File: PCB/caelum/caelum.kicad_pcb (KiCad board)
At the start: 2 copper layers, 48 x 37 mm, 18 parts, among them J1 BATT+, J2 BATT-, J5 PulseIN, J6 PulseOUT, J7 Conn_01x04_Pin, Q1 FS8205A, U1 DW01A, U2 MCP1700T-3302E, U3 ESP32-H2-SUPERMINI

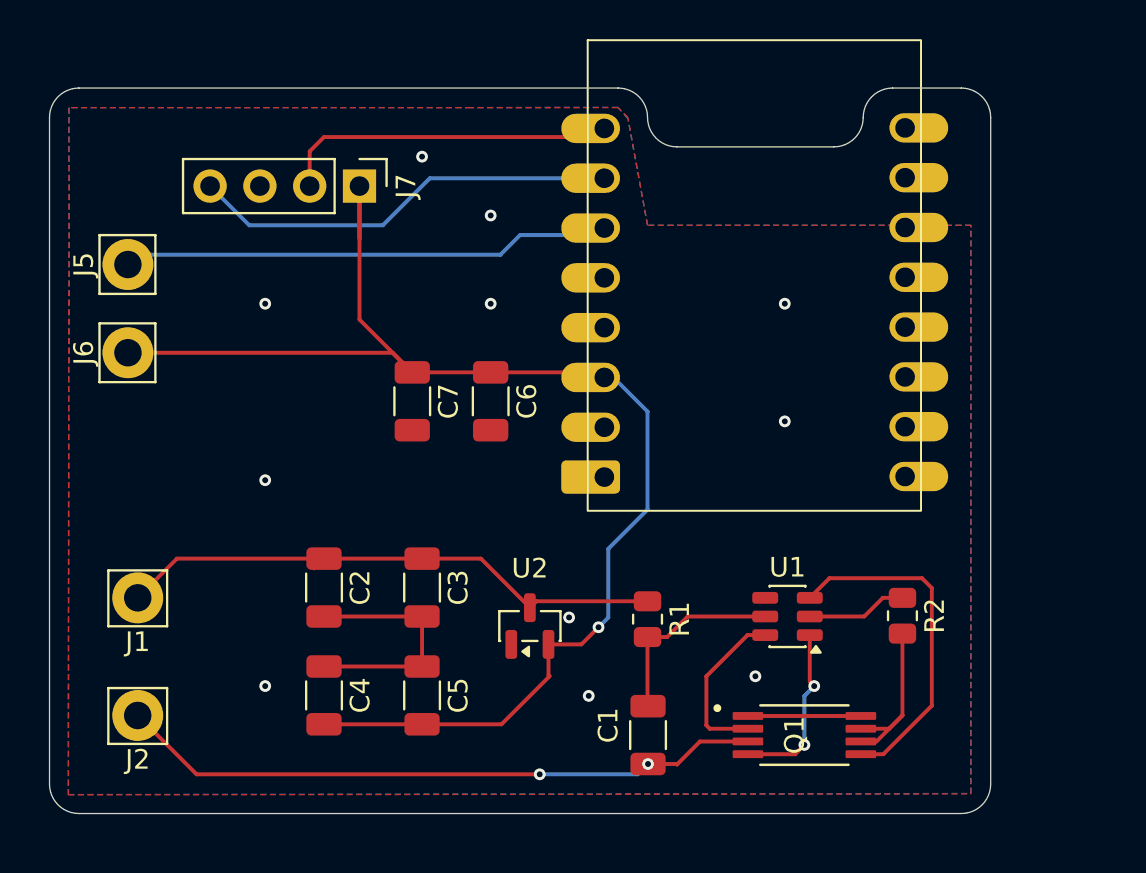
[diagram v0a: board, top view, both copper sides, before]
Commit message: PCB version 1.0
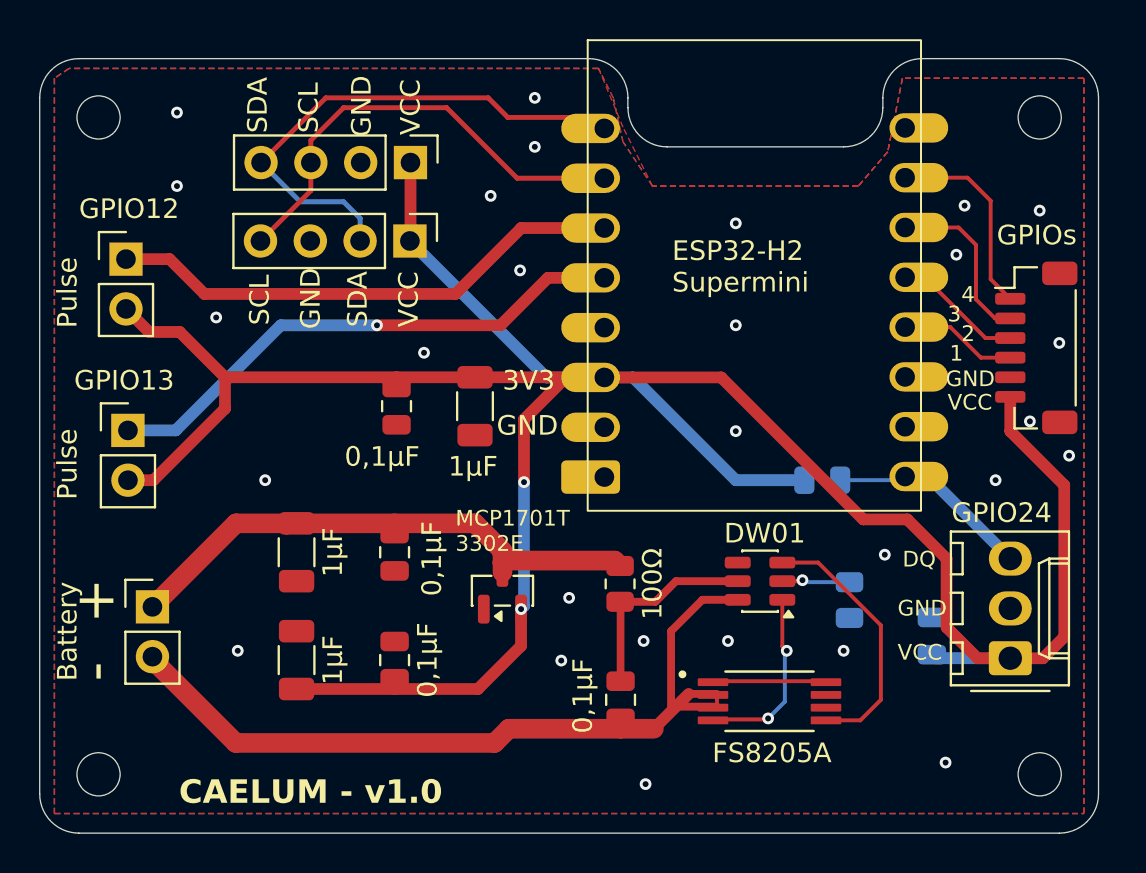
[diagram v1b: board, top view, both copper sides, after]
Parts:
- removed J2: BATT-, Connector_Pin:Pin_D1.4mm_L8.5mm_W2.8mm_FlatFork
- removed J5: PulseIN, Connector_Pin:Pin_D1.4mm_L8.5mm_W2.8mm_FlatFork
- added 0,1µF: 0.1µF, Capacitor_SMD:C_0805_2012Metric, B.Cu at (102.5, 56.0)
- added H1: MountingHole, MountingHole:MountingHole_2.2mm_M2, F.Cu at (60.0, 29.5)
- added H2: MountingHole, MountingHole:MountingHole_2.2mm_M2, F.Cu at (60.0, 63.0)
- added H3: MountingHole, MountingHole:MountingHole_2.2mm_M2, F.Cu at (108.0, 29.5)
- added H4: MountingHole, MountingHole:MountingHole_2.2mm_M2, F.Cu at (108.0, 63.0)
- added J10: Conn_01x04_Pin, Connector_PinHeader_2.54mm:PinHeader_1x04_P2.54mm_Vertical, F.Cu at (75.9, 31.8)
- added J3: Pulse1, Connector_PinHeader_2.54mm:PinHeader_1x02_P2.54mm_Vertical, F.Cu at (61.4, 36.7)
- added J4: Batt, Connector_PinHeader_2.54mm:PinHeader_1x02_P2.54mm_Vertical, F.Cu at (62.8, 54.5)
- added J8: DS18B20, Connector_Molex:Molex_KK-254_AE-6410-03A_1x03_P2.54mm_Vertical, F.Cu at (106.5, 57.1)
- added R3: 4.7KΩ, Resistor_SMD:R_0805_2012Metric, B.Cu at (96.9, 48.0)
- 0,1µF: renamed from C7; footprint Capacitor_SMD:C_1206_3216Metric -> Capacitor_SMD:C_0805_2012Metric
- 0,1µF: renamed from C5; footprint Capacitor_SMD:C_1206_3216Metric -> Capacitor_SMD:C_0805_2012Metric
- 0,1µF: renamed from C1; footprint Capacitor_SMD:C_1206_3216Metric -> Capacitor_SMD:C_0805_2012Metric
- 0,1µF: renamed from C3; footprint Capacitor_SMD:C_1206_3216Metric -> Capacitor_SMD:C_0805_2012Metric
- 1KΩ: renamed from R2; moved to B.Cu
- J1: value BATT+ -> Conn_01x06_Pin; footprint Connector_Pin:Pin_D1.4mm_L8.5mm_W2.8mm_FlatFork -> Connector_JST:JST_SH_BM06B-SRSS-TB_1x06-1MP_P1.00mm_Vertical
- J6: value PulseOUT -> Pulse2; footprint Connector_Pin:Pin_D1.4mm_L8.5mm_W2.8mm_FlatFork -> Connector_PinHeader_2.54mm:PinHeader_1x02_P2.54mm_Vertical
- Q1: value FS8205A -> FS8205A-FC; footprint FS8205A:SOP65P640X120-8N -> FS8205A:SOP65P640X120-8N-FC
- moved J1 47.6 mm to (107.8, 41.2), turned to -90 degrees
- moved J6 3.96 mm to (61.5, 45.5), turned to 0 degrees
- moved J7 3.80 mm to (75.9, 35.8)
- moved 1KΩ 2.82 mm to (98.3, 54.1)
- moved Q1 2.48 mm to (94.2, 59.3)
- moved 0,1µF 2.28 mm to (75.1, 57.2)
- moved 0,1µF 2.28 mm to (75.1, 51.7)
- moved 1µF 2.28 mm to (70.1, 57.2)
- moved 1µF 2.28 mm to (70.1, 51.7)
- moved U1 2.28 mm to (93.7, 53.1)
- moved 0,1µF 2.28 mm to (86.6, 59.2)
- moved 100Ω 2.28 mm to (86.6, 53.3)
- moved U2 2.28 mm to (80.6, 53.6)
- moved 0,1µF 0.84 mm to (75.2, 44.2)
- moved 1µF 0.84 mm to (79.2, 44.2)
- renumbered R1 to 100Ω, C4 to 1µF, C6 to 1µF, C2 to 1µF
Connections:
- J1 pad 1: BATT+ -> GPIO4
- J6 pad 1: +3V3 -> GPIO13
- U3 pad 13: unconnected-(U3-IO4-Pad13) -> GPIO4
- U3 pad 14: unconnected-(U3-IO3-Pad14) -> GPIO3
- U3 pad 15: unconnected-(U3-IO2-Pad15) -> GPIO2
- U3 pad 16: unconnected-(U3-IO1-Pad16) -> GPIO1
- U3 pad 19: unconnected-(U3-IO24-Pad19) -> GPIO24
- U3 pad 5: unconnected-(U3-IO13-Pad5) -> GPIO13
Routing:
- net +3V3: track 70.2 -> 141.4 mm, vias 1 -> 2
- net GPIO13: track 0.00 -> 27.5 mm, vias 0 -> 1
- net OUT-: track 21.8 -> 0.00 mm, vias 11 -> 28
- net GPIO24: track 0.00 -> 10.5 mm
- net GPIO4: track 0.00 -> 10.3 mm
- net SDA: track 17.3 -> 26.9 mm
- net GPIO3: track 0.00 -> 8.91 mm
- net GPIO2: track 0.00 -> 6.65 mm
- net GPIO1: track 0.00 -> 6.01 mm
- net BATT-: track 41.6 -> 46.0 mm, vias 2 -> 0
- net Net-(Q1-G2): track 17.5 -> 13.5 mm
- net Net-(U1-CS): track 5.12 -> 3.49 mm, vias 0 -> 1
- net GPIO12: track 25.1 -> 26.5 mm
- net SCL: track 21.9 -> 23.3 mm
- net BATT+: track 28.7 -> 28.2 mm
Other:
- board size 48 x 37 mm -> 54 x 39.5 mm
- board text added: "+"
- board text added: "-"
- board text added: "1"
- board text added: "2"
- board text added: "3"
- board text added: "3V3"
- board text added: "4"
- board text added: "4.7KΩ"
- board text added: "Battery"
- board text added: "CAELUM - v1.0"
- board text added: "DQ"
- board text added: "DW01"
- board text added: "ESP32-H2 Supermini"
- board text added: "FS8205A"
- board text added: "GND"
- board text added: "GPIO12"
- board text added: "GPIO13"
- board text added: "GPIO24"
- board text added: "GPIOs"
- board text added: "MCP1701T 3302E"
- board text added: "Pulse"
- board text added: "SCL"
- board text added: "SDA"
- board text added: "VCC"
